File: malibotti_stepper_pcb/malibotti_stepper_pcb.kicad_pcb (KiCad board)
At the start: 2 copper layers, 70 x 68 mm, 65 parts, among them J1 Stepper 1, J2 Stepper 1, J3 Servo, J4 Conn_01x04, J5 USB_C_Receptacle_USB2.0_16P, J6 Conn_01x04, SW1 RST, SW2 MicroSwitchLeft, SW3 MicroSwitchRight, SW8 BTN, U1 ESP32-C3-MINI-1, U2 XC6206PxxxMR, U3 STSPIN220, U4 STSPIN220

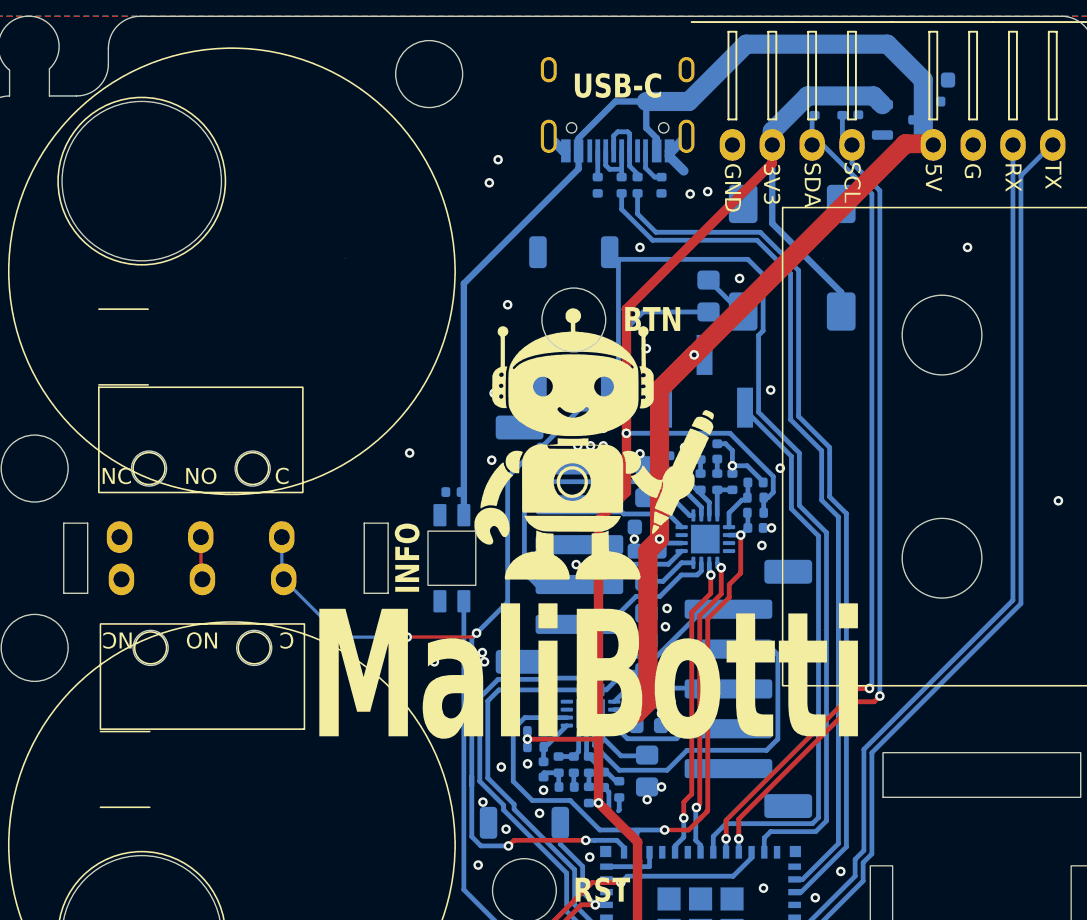
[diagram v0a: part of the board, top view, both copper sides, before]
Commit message: Minor improvements
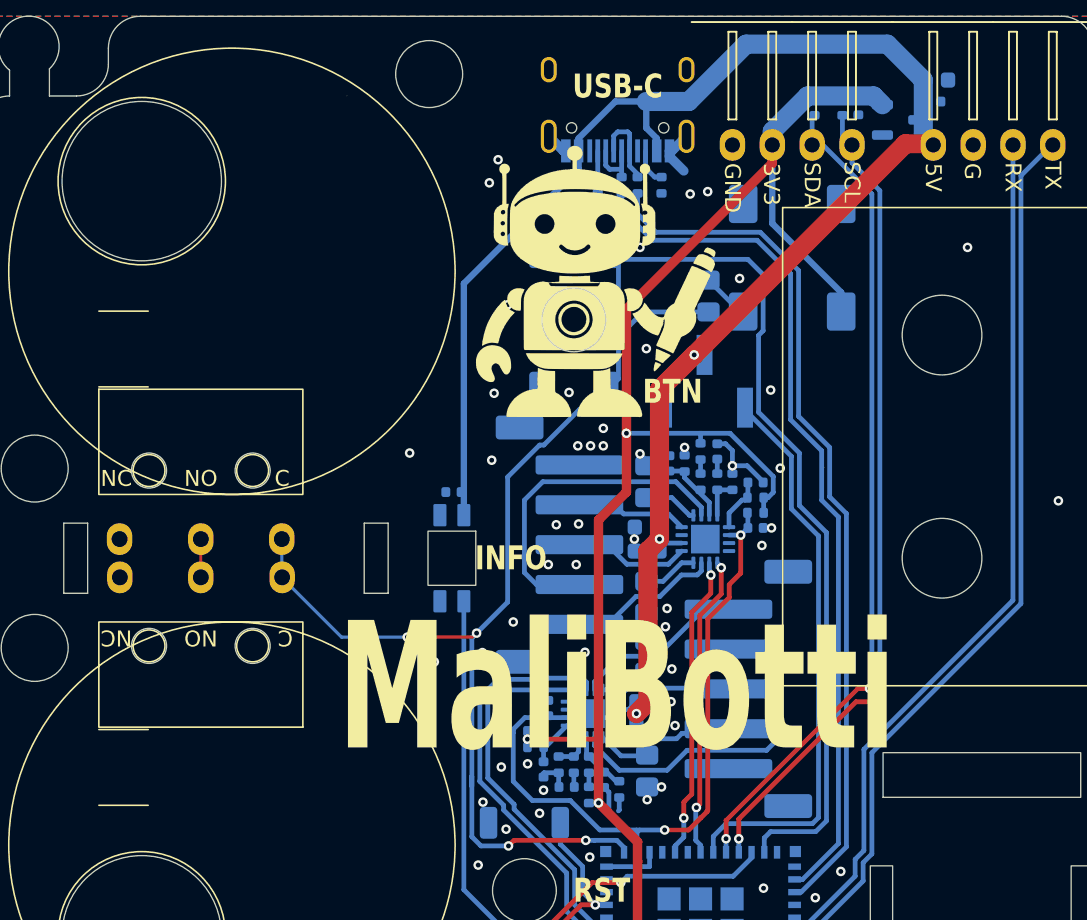
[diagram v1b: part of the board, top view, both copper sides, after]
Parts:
- moved G*** 10.2 mm to (88.2, 82.7)
- moved SW3 0.16 mm to (64.0, 104.0)
- moved SW2 0.12 mm to (64.0, 96.0)
